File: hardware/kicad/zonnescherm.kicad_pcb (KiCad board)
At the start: 2 copper layers, 71.1 x 67.4 mm, 27 parts, among them K1 K1-ON/OFF, K2 K1-UP/DOWN, K3 K2-ON/OFF, K4 K2-UP/DOWN, P1 ARDUINO-ISP, P2 CONN_MAINS, P3 CONN_SUNSHADE1, P4 CONN_SUNSHADE2, P5 SWITCHES, U1 IRM-05-5, U2 LM1117-3.3, U3 ESP-12E, U4 ULN2003A

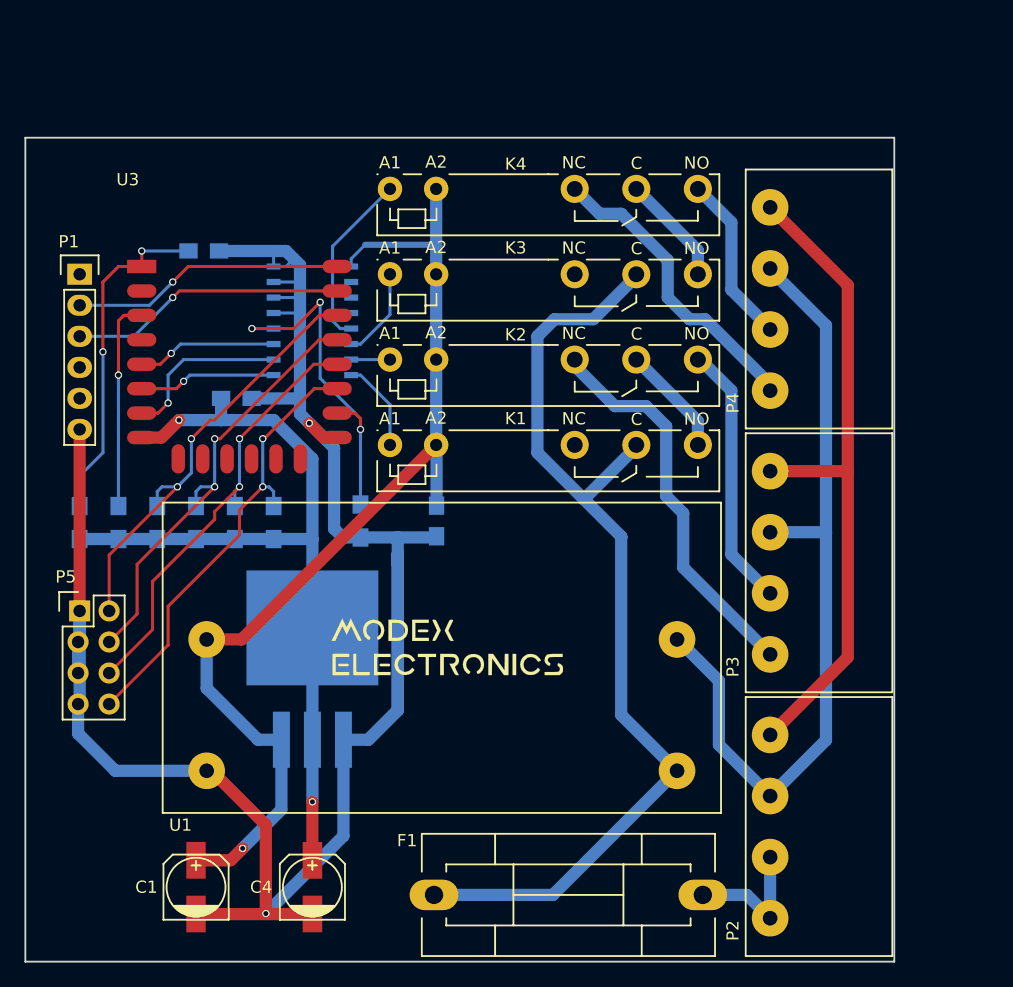
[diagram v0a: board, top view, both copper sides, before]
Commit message: Updated layout, added text etc.
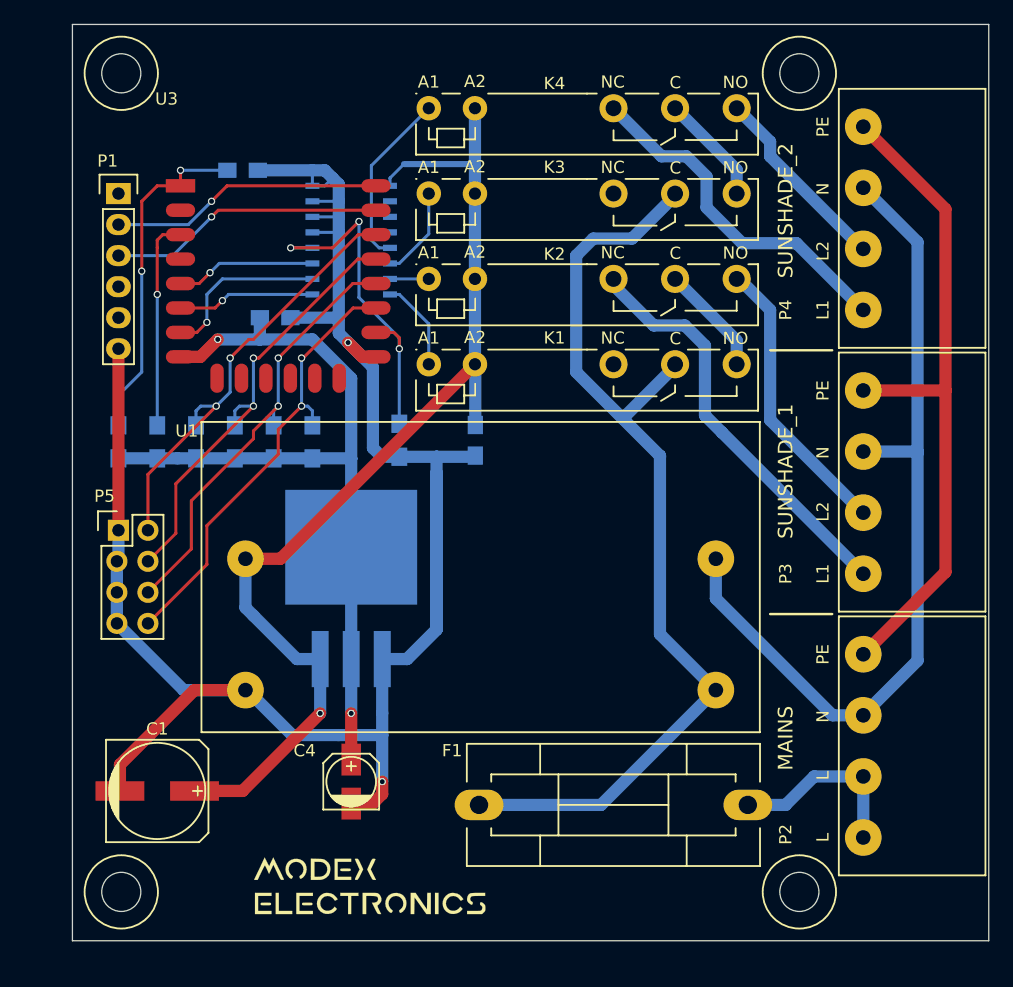
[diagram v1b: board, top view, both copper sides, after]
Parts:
- added REF**: board_75x75_mm, modex:board_75x75_mm_mod, F.Cu at (108.5, 58.9)
- C1: footprint Capacitors_SMD:c_elec_5x5.3 -> Capacitors_SMD:c_elec_8x6.5
- C4: footprint Capacitors_SMD:c_elec_5x5.3 -> Capacitors_SMD:c_elec_4x5.8
- moved G*** 20.6 mm to (132.8, 129.3)
- moved P2 10.1 mm to (173.2, 125.5)
- moved P3 10.1 mm to (173.2, 103.9)
- moved P4 10.1 mm to (173.2, 82.3)
- moved C4 9.20 mm to (131.3, 120.9)
- moved C1 8.49 mm to (115.4, 121.7), turned to 0 degrees
- moved F1 8.24 mm to (152.8, 122.8)
- moved C5 7.33 mm to (141.5, 93.0)
- moved K1 7.33 mm to (137.7, 86.7)
- moved K2 7.33 mm to (137.7, 79.8)
- moved K3 7.33 mm to (137.7, 72.8)
- moved K4 7.33 mm to (137.7, 65.8)
- moved P5 7.33 mm to (112.1, 100.3)
- moved R1 7.33 mm to (121.8, 93.1)
- moved U1 7.33 mm to (161.2, 113.4)
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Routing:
- net GND: track 174.2 -> 168.7 mm
- net Net-(F1-Pad2): track 11.3 -> 15.4 mm
- net Net-(K4-Pad3): track 25.0 -> 28.9 mm
- net N: track 67.8 -> 70.8 mm
- net P5V: track 85.9 -> 88.9 mm
- net Net-(K4-Pad5): track 14.0 -> 15.9 mm
- net Net-(K2-Pad5): track 21.7 -> 23.6 mm
- net Net-(K2-Pad3): track 32.2 -> 34.1 mm
- net P3V3: track 78.6 -> 77.0 mm
- net P: track 81.2 -> 80.3 mm
- net PE: track 54.8 -> 55.5 mm
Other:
- board size 71.1 x 67.4 mm -> 75 x 75 mm
- board text added: "L"
- board text added: "L1"
- board text added: "L2"
- board text added: "MAINS"
- board text added: "N"
- board text added: "PE"
- board text added: "SUNSHADE_1"
- board text added: "SUNSHADE_2"
